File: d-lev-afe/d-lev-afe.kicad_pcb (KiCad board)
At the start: 2 copper layers, 109.4 x 93 mm, 26 parts, among them J1 S8B-PH-SM4-TB, Q1 MMBT3904, Q2 MMBT3906, U1 74AHC04, U2 HT7533-1-SOT89, U3 SRV05-4

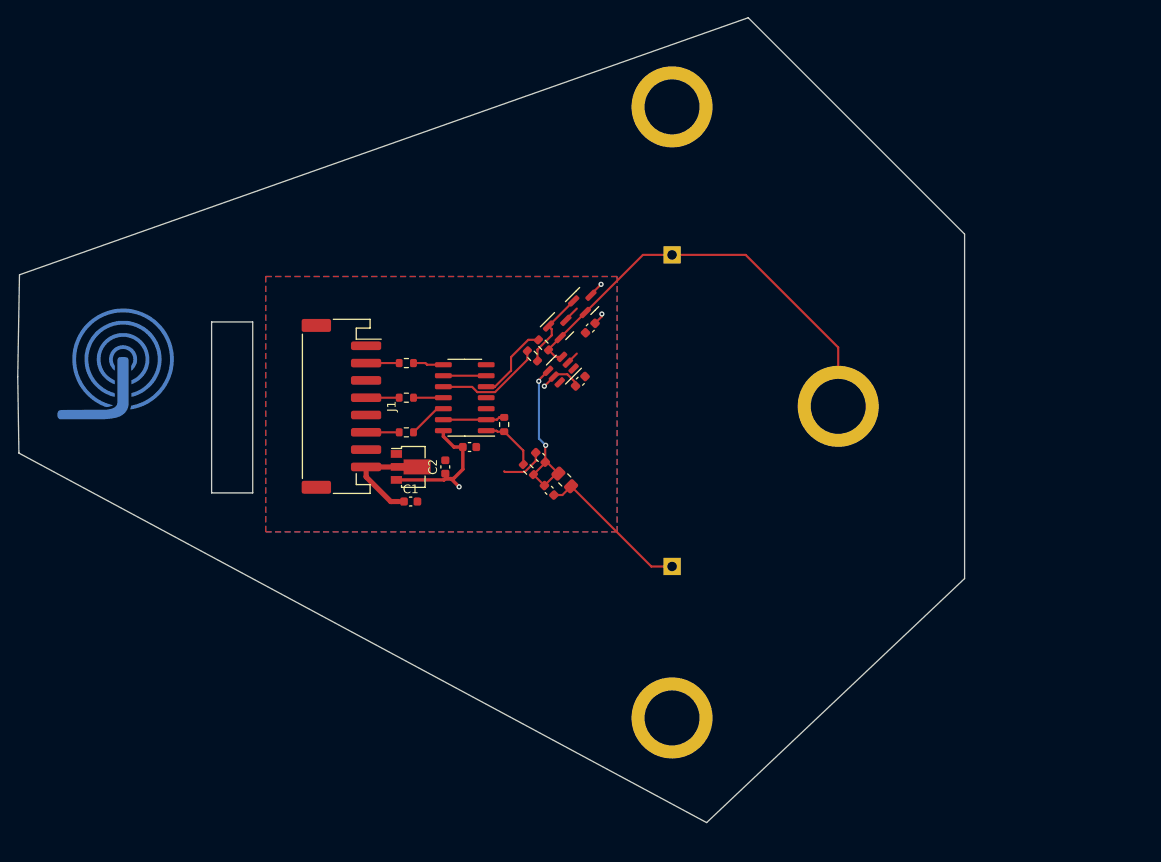
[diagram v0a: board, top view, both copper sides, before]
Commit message: many many changes'
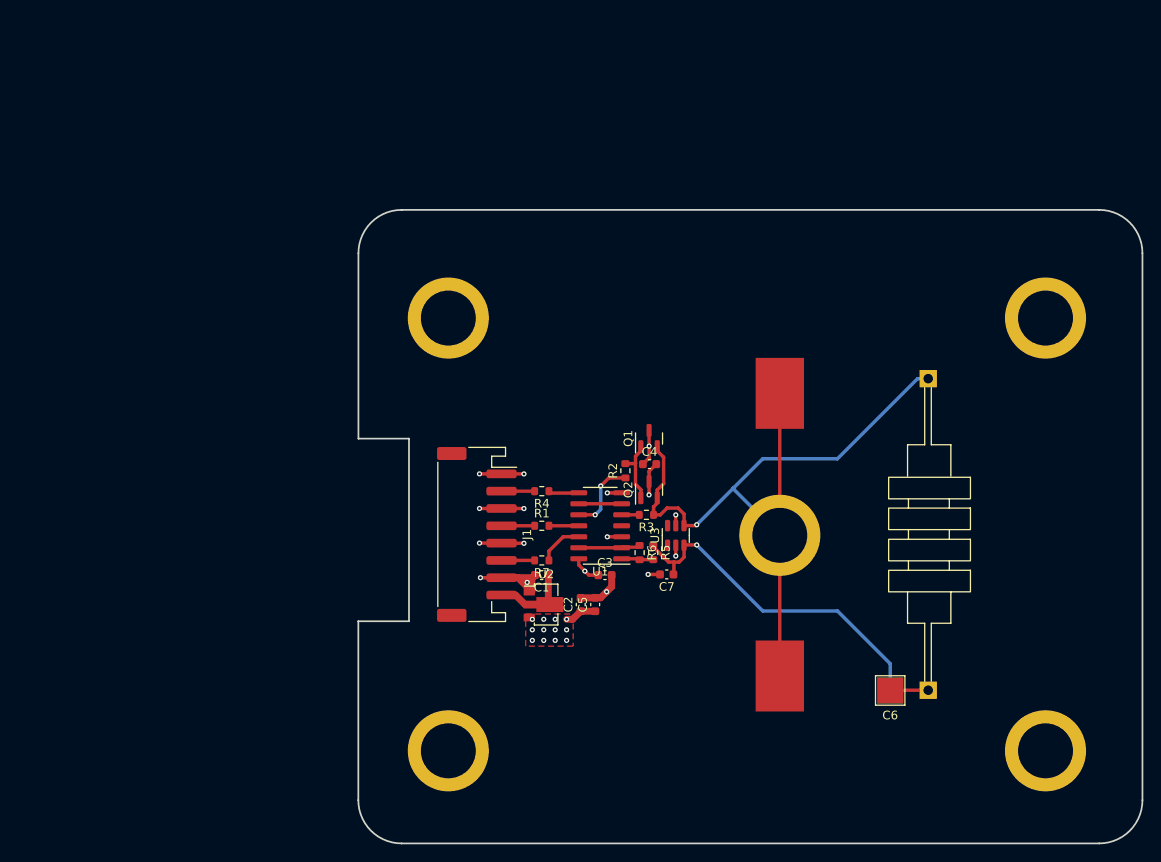
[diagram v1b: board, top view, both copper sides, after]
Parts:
- removed C8: 1p, Capacitor_SMD:C_0805_2012Metric_Pad1.18x1.45mm_HandSolder
- removed G***: LOGO, theremin:logo
- added AE1: PLATE, theremin:keystone-PN5331TR, F.Cu at (181.3, 107.5)
- added AE2: PLATE, theremin:keystone-PN5331TR, F.Cu at (181.3, 82.5)
- added H4: Standoff_2, theremin:SMTSO-M4, F.Cu at (212.0, 70.0)
- added H5: Standoff_2, theremin:SMTSO-M4, F.Cu at (212.0, 120.0)
- C6: footprint Capacitor_SMD:C_0603_1608Metric -> theremin:testpoint_cap_1pf
- H1, H2, H3, L1: moved to F.Cu
- J1: footprint Connector_JST:JST_PH_S8B-PH-SM4-TB_1x08-1MP_P2.00mm_Horizontal -> theremin:JST_PH_S8B-PH-SM4-TB_1x08-1MP_P2.00mm_Horizontal
- moved H3 78.8 mm to (143.0, 120.0), turned to 0 degrees
- moved C6 45.7 mm to (194.1, 113.0), turned to 180 degrees
- moved H2 44.5 mm to (143.0, 70.0), turned to 0 degrees
- moved L1 32.9 mm to (198.4, 95.0)
- moved C5 25.9 mm to (160.0, 103.1), turned to 90 degrees
- moved U3 23.3 mm to (169.3, 95.1), turned to 90 degrees
- moved R3 23.0 mm to (165.9, 92.7), turned to 180 degrees
- moved C2 22.3 mm to (158.3, 103.1)
- moved U2 22.3 mm to (154.3, 103.1)
- moved C3 21.5 mm to (161.1, 99.7)
- moved J1 21.5 mm to (146.3, 95.0)
- moved R1 21.5 mm to (153.8, 94.0)
- moved R4 21.5 mm to (153.8, 90.0)
- moved R6 21.5 mm to (165.1, 97.1)
- moved R7 21.5 mm to (153.8, 98.0)
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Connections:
- U3 pad 3: L_OUT -> /C_DIV
- U3 pad 4: /C_DIV -> L_OUT
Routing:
- net L_OUT: track 51.2 -> 89.1 mm, vias 0 -> 1
- net GND: track 8.54 -> 42.3 mm, vias 0 -> 14
- net /C_DIV: track 19.4 -> 40.1 mm, vias 2 -> 1
- net L_IN: track 17.9 -> 4.40 mm
- net +3V3: track 24.3 -> 12.8 mm, vias 4 -> 15
- net Net-(R3-Pad2): track 9.78 -> 2.04 mm
- net Net-(R2-Pad1): track 12.5 -> 8.73 mm, vias 0 -> 2
- net Net-(R5-Pad2): track 6.85 -> 3.70 mm
- net +5V: track 9.72 -> 7.20 mm
- net Net-(Q1-B): track 8.97 -> 7.62 mm
- net Net-(R7-Pad1): track 4.58 -> 5.22 mm
- added copper zone on F.Cu, net +3V3
- added copper zone on In2.Cu, net +3V3
- added copper zone on In1.Cu, net GND
- removed copper zone on B.Cu, net +3V3
- removed copper zone on F.Cu, net GND
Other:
- board size 109.4 x 93 mm -> 90.6 x 73.2 mm
- copper layers 2 -> 4
- rule solder_mask_min_width: 0.2 -> 0.15
- board text removed: "L_OUT Drive side - near antenna mount"
- board text removed: "Sense side Minimize copper"
